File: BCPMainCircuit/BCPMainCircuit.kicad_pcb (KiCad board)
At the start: 2 copper layers, 94 x 88 mm, 14 parts, among them SW1 Switch, U1 3.3 Volt Regulator, U2 Pico 2, U3 Logger, U5 BNO055, U6 BME280

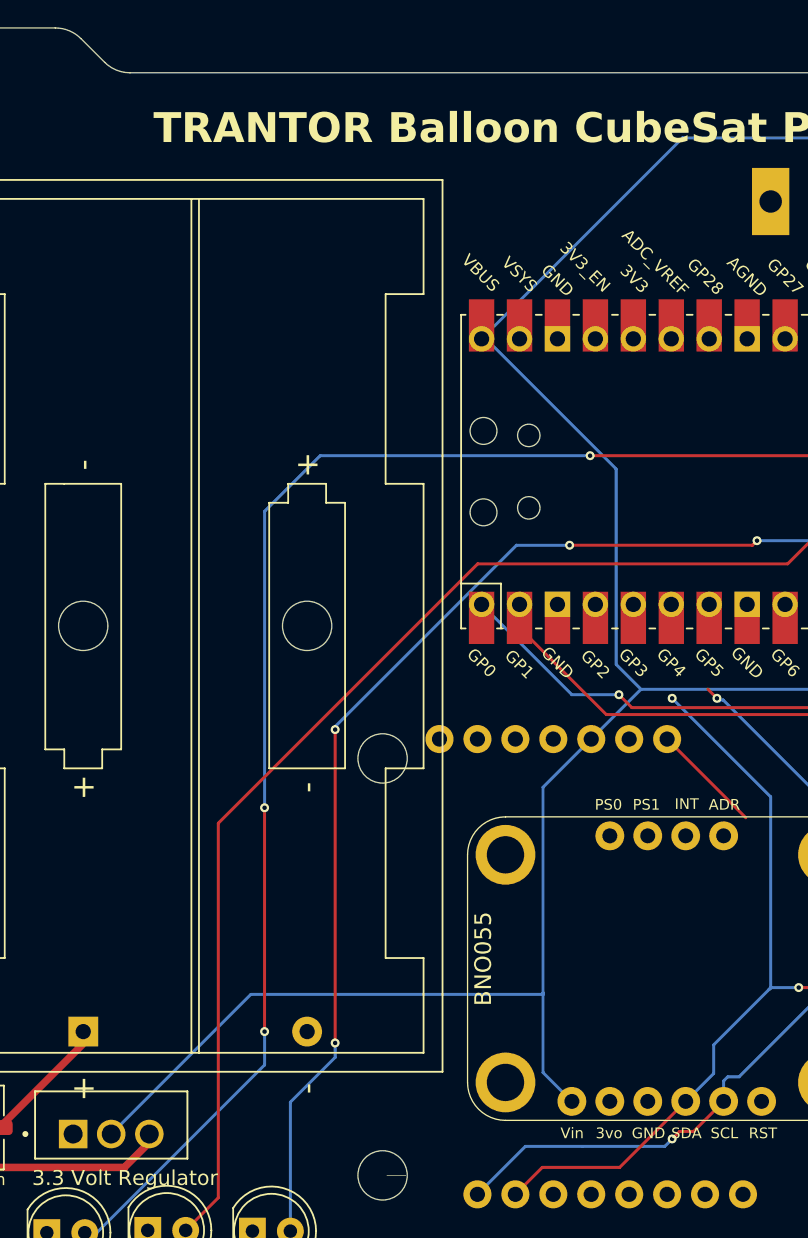
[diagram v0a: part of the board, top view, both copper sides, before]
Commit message: Update PCB design
Added four new backup ZIP files for BCPMainCircuit. Updated the KiCad PCB file to include a detailed stackup and new F.SilkS graphics, and made related changes to the .kicad_prl and fp-info-cache files.
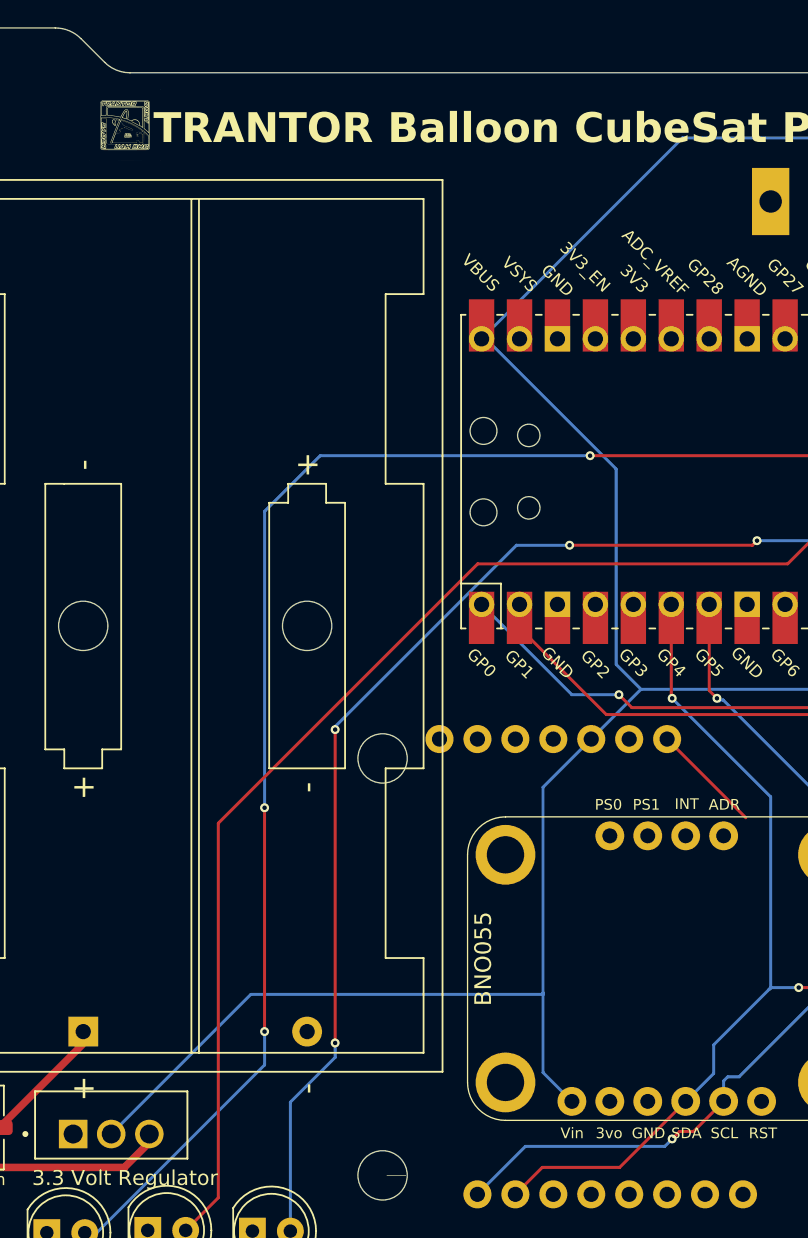
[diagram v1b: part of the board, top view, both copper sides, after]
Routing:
- net /SDA: track 66.7 -> 72.8 mm
- net /SCL: track 72.2 -> 77.8 mm
